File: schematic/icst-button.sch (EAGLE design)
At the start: 4 parts

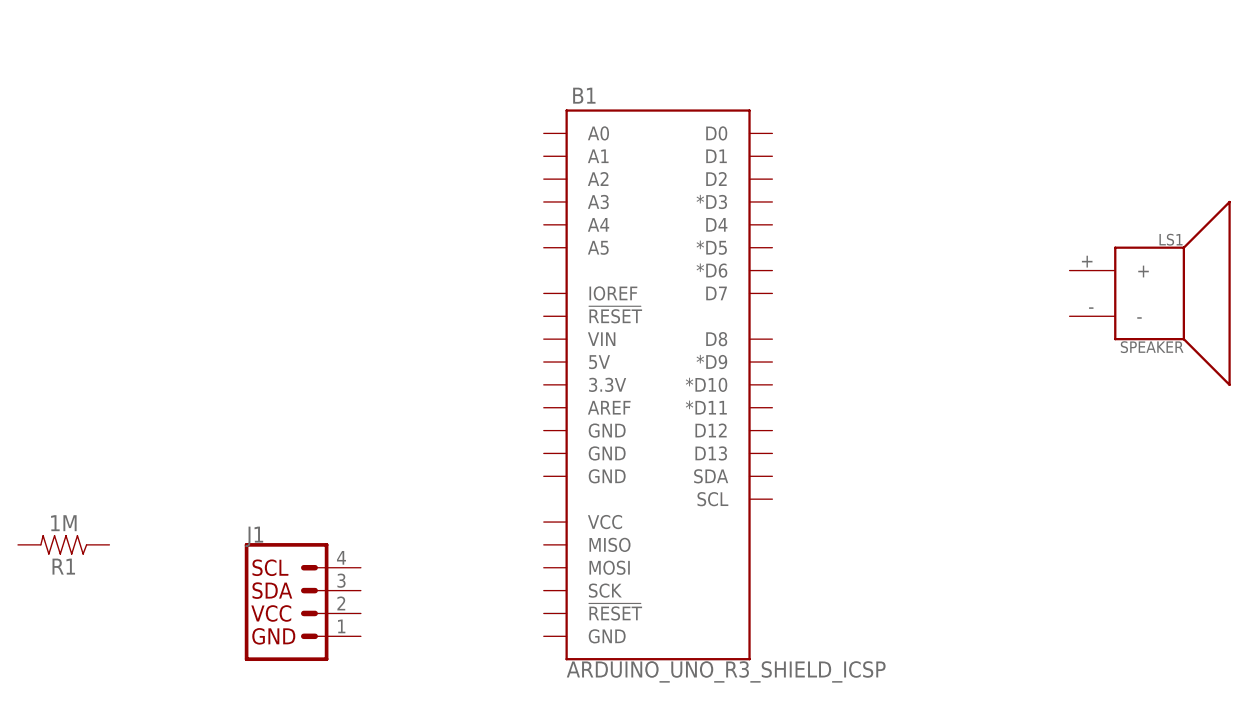
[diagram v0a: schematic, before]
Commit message: compeleted schematic
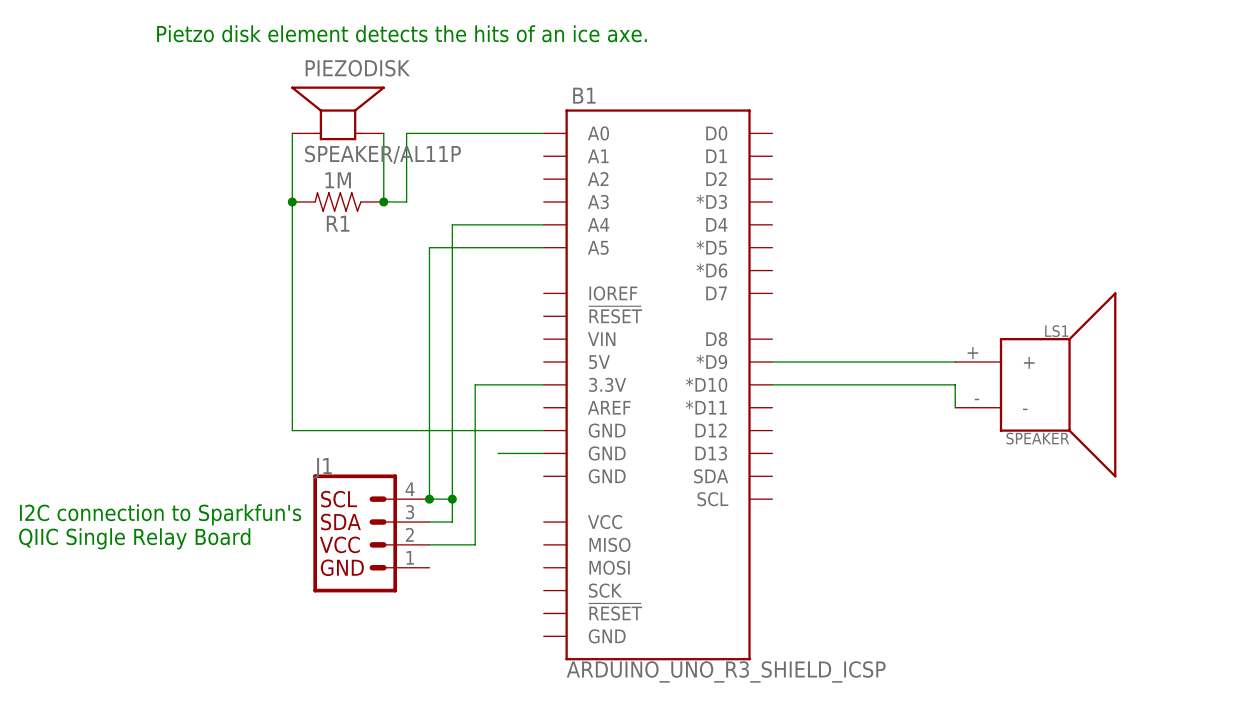
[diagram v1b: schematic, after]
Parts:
- added PIEZODISK: SPEAKER/AL11P, adafruit:SPEAKER/AL11P
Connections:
- new net N$1: B1.*D9, LS1.+
- new net N$2: B1.*D10, LS1.-
- new net N$3: B1.GND@2, PIEZODISK.+, R1.2
- new net N$4: B1.A0, PIEZODISK.-, R1.1
- new net N$5: B1.A4, B1.A5, J1.SCL, J1.SDA
- new net N$7: B1.3.3V, J1.VCC
- new net N$8: B1.GND@1
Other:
- note added: "I2C connection to Sparkfun's QIIC Single Relay Board"
- note added: "Pietzo disk element detects the hits of an ice axe."
- moved on the sheet: J1, LS1, R1
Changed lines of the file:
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@@
 <layer number="230" name="230bmp" color="7" fill="1" visible="yes" active="yes"/>
 <layer number="231" name="231bmp" color="7" fill="1" visible="yes" active="yes"/>
+<layer number="232" name="Eagle3D_PG2" color="7" fill="1" visible="no" active="no"/>
+<layer number="233" name="Eagle3D_PG3" color="7" fill="1" visible="no" active="no"/>
 <layer number="248" name="Housing" color="7" fill="1" visible="yes" active="yes"/>
 <layer number="249" name="Edge" color="7" fill="1" visible="yes" active="yes"/>
@@
 <part name="R1" library="SparkFun-Resistors" library_urn="urn:adsk.eagle:library:532" deviceset="1MOHM" device="-0603-1/4W-5%" package3d_urn="urn:adsk.eagle:package:39650/1" value="1M"/>
 <part name="J1" library="SparkFun-Connectors" library_urn="urn:adsk.eagle:library:513" deviceset="QWIIC_CONNECTOR" device="JS-1MM" package3d_urn="urn:adsk.eagle:package:38096/1"/>
+<part name="PIEZODISK" library="adafruit" library_urn="urn:adsk.eagle:library:420" deviceset="SPEAKER" device="/AL11P" package3d_urn="urn:adsk.eagle:package:6240662/1"/>
 </parts>
 <sheets>
 <sheet>
 <plain>
+<text x="20.32" y="93.98" size="1.778" layer="91">Pietzo disk element detects the hits of an ice axe.</text>
+<text x="5.08" y="38.1" size="1.778" layer="91">I2C connection to Sparkfun's
+QIIC Single Relay Board</text>
 </plain>
 <instances>
@@
 <attribute name="VALUE" x="66.04" y="25.146" size="1.778" layer="96" font="vector" align="top-left"/>
 </instance>
-<instance part="LS1" gate="G$1" x="132.08" y="66.04" smashed="yes">
-<attribute name="NAME" x="134.62" y="71.374" size="1.27" layer="95" font="vector" rot="MR0"/>
-<attribute name="VALUE" x="134.62" y="60.706" size="1.27" layer="96" font="vector" rot="R180"/>
+<instance part="LS1" gate="G$1" x="119.38" y="55.88" smashed="yes">
+<attribute name="NAME" x="121.92" y="61.214" size="1.27" layer="95" font="vector" rot="MR0"/>
+<attribute name="VALUE" x="121.92" y="50.546" size="1.27" layer="96" font="vector" rot="R180"/>
 </instance>
-<instance part="R1" gate="G$1" x="10.16" y="38.1" smashed="yes" rot="R180">
-<attribute name="NAME" x="10.16" y="36.576" size="1.778" layer="95" font="vector" rot="R180" align="bottom-center"/>
-<attribute name="VALUE" x="10.16" y="39.624" size="1.778" layer="96" font="vector" rot="R180" align="top-center"/>
+<instance part="R1" gate="G$1" x="40.64" y="76.2" smashed="yes" rot="R180">
+<attribute name="NAME" x="40.64" y="74.676" size="1.778" layer="95" font="vector" rot="R180" align="bottom-center"/>
+<attribute name="VALUE" x="40.64" y="77.724" size="1.778" layer="96" font="vector" rot="R180" align="top-center"/>
 </instance>
-<instance part="J1" gate="J1" x="35.56" y="30.48" smashed="yes">
-<attribute name="VALUE" x="30.48" y="25.146" size="1.778" layer="96" font="vector" align="top-left"/>
-<attribute name="NAME" x="30.48" y="38.354" size="1.778" layer="95" font="vector"/>
+<instance part="J1" gate="J1" x="43.18" y="38.1" smashed="yes">
+<attribute name="VALUE" x="38.1" y="32.766" size="1.778" layer="96" font="vector" align="top-left"/>
+<attribute name="NAME" x="38.1" y="45.974" size="1.778" layer="95" font="vector"/>
+</instance>
+<instance part="PIEZODISK" gate="S1" x="40.64" y="83.82" smashed="yes">
+<attribute name="NAME" x="36.83" y="90.17" size="1.778" layer="95"/>
+<attribute name="VALUE" x="36.83" y="80.645" size="1.778" layer="96"/>
 </instance>
 </instances>
@@
 </busses>
 <nets>
+<net name="N$1" class="0">
+<segment>
+<pinref part="B1" gate="G$1" pin="*D9"/>
+<pinref part="LS1" gate="G$1" pin="+"/>
+<wire x1="88.9" y1="58.42" x2="109.22" y2="58.42" width="0.1524" layer="91"/>
+</segment>
+</net>
+<net name="N$2" class="0">
+<segment>
+<pinref part="B1" gate="G$1" pin="*D10"/>
+<pinref part="LS1" gate="G$1" pin="-"/>
+<wire x1="88.9" y1="55.88" x2="109.22" y2="55.88" width="0.1524" layer="91"/>
+<wire x1="109.22" y1="55.88" x2="109.22" y2="53.34" width="0.1524" layer="91"/>
+</segment>
+</net>
+<net name="N$3" class="0">
+<segment>
+<pinref part="PIEZODISK" gate="S1" pin="+"/>
+<pinref part="R1" gate="G$1" pin="2"/>
+<wire x1="35.56" y1="83.82" x2="35.56" y2="76.2" width="0.1524" layer="91"/>
+<pinref part="B1" gate="G$1" pin="GND@2"/>
+<wire x1="35.56" y1="76.2" x2="35.56" y2="50.8" width="0.1524" layer="91"/>
+<wire x1="35.56" y1="50.8" x2="63.5" y2="50.8" width="0.1524" layer="91"/>
+<junction x="35.56" y="76.2"/>
+</segment>
+</net>
+<net name="N$4" class="0">
+<segment>
+<pinref part="PIEZODISK" gate="S1" pin="-"/>
+<pinref part="R1" gate="G$1" pin="1"/>
+<wire x1="45.72" y1="83.82" x2="45.72" y2="76.2" width="0.1524" layer="91"/>
+<pinref part="B1" gate="G$1" pin="A0"/>
+<wire x1="63.5" y1="83.82" x2="48.26" y2="83.82" width="0.1524" layer="91"/>
+<wire x1="48.26" y1="83.82" x2="48.26" y2="76.2" width="0.1524" layer="91"/>
+<wire x1="48.26" y1="76.2" x2="45.72" y2="76.2" width="0.1524" layer="91"/>
+<junction x="45.72" y="76.2"/>
+</segment>
+</net>
+<net name="N$5" class="0">
+<segment>
+<pinref part="B1" gate="G$1" pin="A4"/>
+<wire x1="63.5" y1="73.66" x2="53.34" y2="73.66" width="0.1524" layer="91"/>
+<pinref part="J1" gate="J1" pin="SDA"/>
+<wire x1="53.34" y1="73.66" x2="53.34" y2="43.18" width="0.1524" layer="91"/>
+<wire x1="53.34" y1="43.18" x2="53.34" y2="40.64" width="0.1524" layer="91"/>
+<wire x1="53.34" y1="40.64" x2="50.8" y2="40.64" width="0.1524" layer="91"/>
+<pinref part="B1" gate="G$1" pin="A5"/>
+<wire x1="63.5" y1="71.12" x2="50.8" y2="71.12" width="0.1524" layer="91"/>
+<wire x1="50.8" y1="71.12" x2="50.8" y2="43.18" width="0.1524" layer="91"/>
+<wire x1="50.8" y1="43.18" x2="53.34" y2="43.18" width="0.1524" layer="91"/>
+<junction x="53.34" y="43.18"/>
+<pinref part="J1" gate="J1" pin="SCL"/>
+<junction x="50.8" y="43.18"/>
+</segment>
+</net>
+<net name="N$7" class="0">
+<segment>
+<pinref part="B1" gate="G$1" pin="3.3V"/>
+<wire x1="63.5" y1="55.88" x2="55.88" y2="55.88" width="0.1524" layer="91"/>
+<pinref part="J1" gate="J1" pin="VCC"/>
+<wire x1="55.88" y1="55.88" x2="55.88" y2="38.1" width="0.1524" layer="91"/>
+<wire x1="55.88" y1="38.1" x2="50.8" y2="38.1" width="0.1524" layer="91"/>
+</segment>
+</net>
+<net name="N$8" class="0">
+<segment>
+<pinref part="B1" gate="G$1" pin="GND@1"/>
+<wire x1="63.5" y1="48.26" x2="58.42" y2="48.26" width="0.1524" layer="91"/>
+</segment>
+</net>
 </nets>
 </sheet>
@@
 </drawing>
 <compatibility>
+<note version="6.3" minversion="6.2.2" severity="warning">
+Since Version 6.2.2 text objects can contain more than one line,
+which will not be processed correctly with this version.
+</note>
 <note version="8.2" severity="warning">
 Since Version 8.2, EAGLE supports online libraries. The ids
